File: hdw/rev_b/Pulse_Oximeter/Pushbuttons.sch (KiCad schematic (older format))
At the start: 12 parts, among them SW1702 Cap_Touch, U1702 TPS71530, U1704 AT42QT1010-TSHR, U1706 74LVC1G17

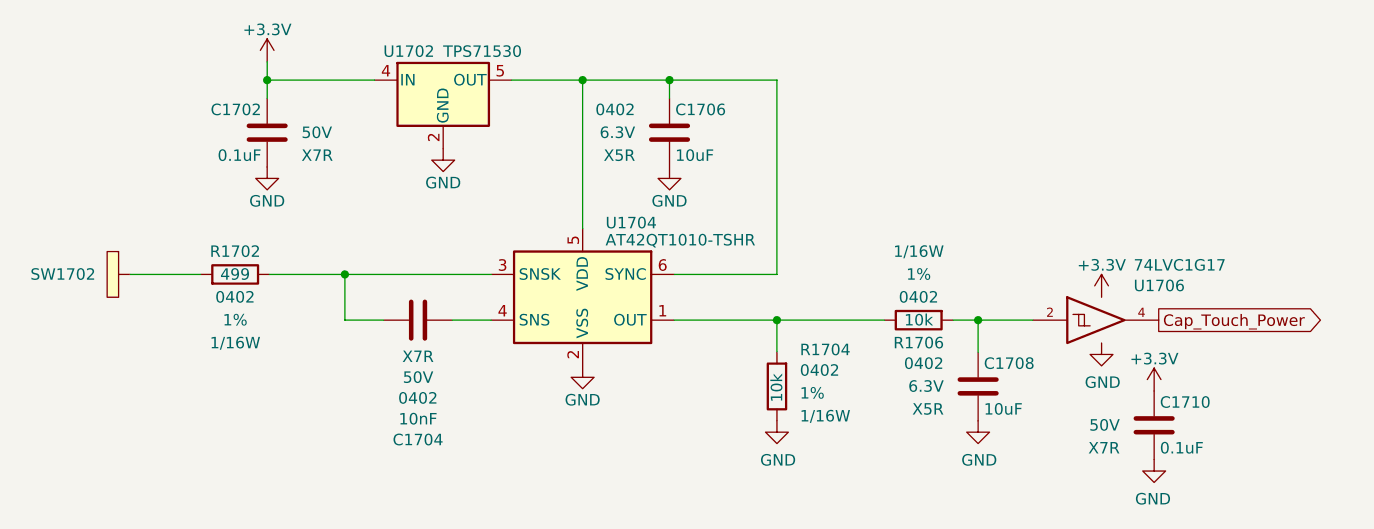
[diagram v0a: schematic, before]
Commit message: change pushbutton sheet
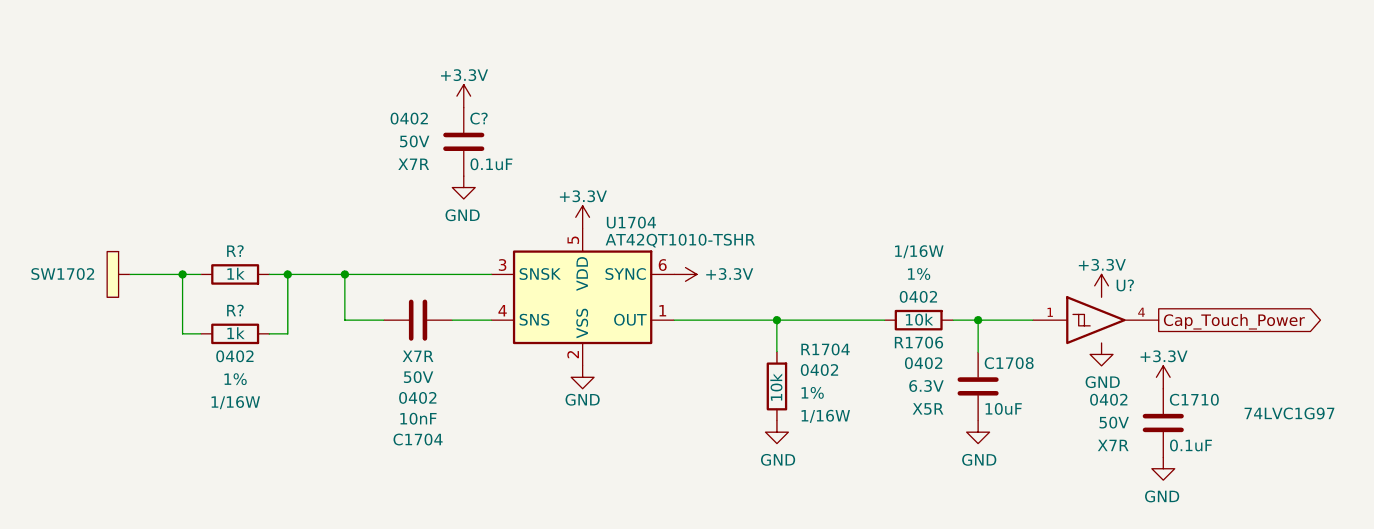
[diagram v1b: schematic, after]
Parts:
- removed C1702: 0.1uF, Capacitors_SMD:C_0402, symbol Custom_Library:C_Custom
- removed C1706: 10uF, Capacitors_SMD:C_0402, symbol Custom_Library:C_Custom
- removed R1702: 499, Resistors_SMD:R_0402, symbol Custom_Library:R_Custom
- removed U1702: TPS71530, Package_TO_SOT_SMD:SOT-353_SC-70-5, symbol Regulator_Linear:TPS71530__SC70
- removed U1706: 74LVC1G17, TO_SOT_Packages_SMD:SOT-353_SC-70-5, symbol Custom_Library:74LVC1G17_Power
- added C?: 0.1uF, Capacitors_SMD:C_0402, symbol Custom_Library:C_Custom
- added R? (x2): 1k, Resistors_SMD:R_0402, symbol Custom_Library:R_Custom
- added U?: 74LVC1G97, Package_TO_SOT_SMD:SOT-363_SC-70-6, symbol Custom_Library:74LVC1G97_Power_BUF
- C1710: display_footprint (none) -> 0402
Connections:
- net +3V3: now also U1704.5 (VDD), U1704.6 (SYNC), C?.1, U?.5 (VCC)
- net Cap_Touch_Power: now also U?.4
- net GND: now also C?.2, U?.2 (GND), U?.3 (GND), U?.6 (GND)
- net at C1704.2, U1704.3 (SNSK): now also R?.1, R?.1
- net at SW1702.1 (TP): now also R?.2, R?.2
- net at C1708.1, R1706.1: now also U?.1
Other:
- moved on the sheet: C1710

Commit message: changed all passives to 0402, cleared digikey pns
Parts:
- C1704: Digi-Key PN 490-13295-1-ND -> (none)
- C1708: Digi-Key PN 490-13211-1-ND -> (none)
- C1710, C?: Digi-Key PN 490-10701-1-ND -> (none)
- R1704, R1706: Digi-Key PN RMCF0402FT10K0CT-ND -> (none)
- R? (x2): Digi-Key PN 541-1.00KLCT-ND -> (none)
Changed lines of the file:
@@
 F 2 "Capacitors_SMD:C_0402" H 4038 2310 50  0001 C CNN
 F 3 "" H 4025 2560 50  0001 C CNN
-F 4 "490-13295-1-ND" H -790 240 50  0001 C CNN "Digi-Key PN"
+F 4 "" H -790 240 50  0001 C CNN "Digi-Key PN"
 F 5 "0402" V 3658 2460 50  0000 C CNN "display_footprint"
 F 6 "50V" V 3749 2460 50  0000 C CNN "Voltage"
@@
 F 5 "1%" H 5670 2720 50  0000 L CNN "Tolerance"
 F 6 "1/16W" H 5670 2620 50  0000 L CNN "Wattage"
-F 7 "RMCF0402FT10K0CT-ND" H 5870 3150 60  0001 C CNN "Digi-Key PN"
+F 7 "" H 5870 3150 60  0001 C CNN "Digi-Key PN"
 	1    5570 2750
 	1    0    0    -1
@@
 F 5 "1%" V 6390 2460 50  0000 C CNN "Tolerance"
 F 6 "1/16W" V 6490 2460 50  0000 C CNN "Wattage"
-F 7 "RMCF0402FT10K0CT-ND" H 6190 2460 50  0001 C CNN "Digi-Key PN"
+F 7 "" H 6190 2460 50  0001 C CNN "Digi-Key PN"
 	1    6190 2460
 	0    1    -1   0
@@
 F 2 "Capacitors_SMD:C_0402" H 7298 2760 50  0001 C CNN
 F 3 "" H 7285 3010 50  0001 C CNN
-F 4 "490-10701-1-ND" H 7685 3410 60  0001 C CNN "Digi-Key PN"
+F 4 "" H 7685 3410 60  0001 C CNN "Digi-Key PN"
 F 5 "0402" H 7110 3010 50  0000 R CNN "display_footprint"
 F 6 "50V" H 7110 2910 50  0000 R CNN "Voltage"
@@
 F 5 "6.3V" H 6300 2750 50  0000 R CNN "Voltage"
 F 6 "X5R" H 6300 2650 50  0000 R CNN "Dielectric"
-F 7 "490-13211-1-ND" H 6450 2750 50  0001 C CNN "Digi-Key PN"
+F 7 "" H 6450 2750 50  0001 C CNN "Digi-Key PN"
 	1    6450 2750
 	1    0    0    -1
@@
 F 2 "Capacitors_SMD:C_0402" H 4238 1530 50  0001 C CNN
 F 3 "" H 4225 1780 50  0001 C CNN
-F 4 "490-10701-1-ND" H 4625 2180 60  0001 C CNN "Digi-Key PN"
+F 4 "" H 4625 2180 60  0001 C CNN "Digi-Key PN"
 F 5 "0402" H 4050 1780 50  0000 R CNN "display_footprint"
 F 6 "50V" H 4050 1680 50  0000 R CNN "Voltage"
@@
 F 5 "1%" V 3400 2260 50  0001 C CNN "Tolerance"
 F 6 "1/16W" V 3500 2260 50  0001 C CNN "Wattage"
-F 7 "541-1.00KLCT-ND" H 3500 2660 60  0001 C CNN "Digi-Key PN"
+F 7 "" H 3500 2660 60  0001 C CNN "Digi-Key PN"
 	1    3200 2260
 	0    1    1    0
@@
 F 5 "1%" V 3400 2520 50  0000 C CNN "Tolerance"
 F 6 "1/16W" V 3500 2520 50  0000 C CNN "Wattage"
-F 7 "541-1.00KLCT-ND" H 3500 2920 60  0001 C CNN "Digi-Key PN"
+F 7 "" H 3500 2920 60  0001 C CNN "Digi-Key PN"
 	1    3200 2520
 	0    1    1    0
